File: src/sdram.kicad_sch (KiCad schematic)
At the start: 8 parts, among them U1 ECP5U_12_CABGA256, U10 W9825G6KH-6

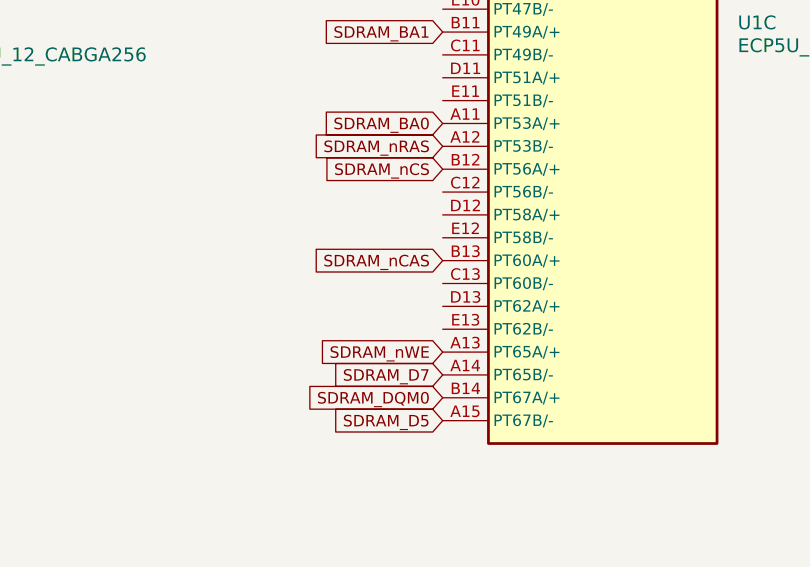
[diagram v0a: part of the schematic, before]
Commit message: Rev 2
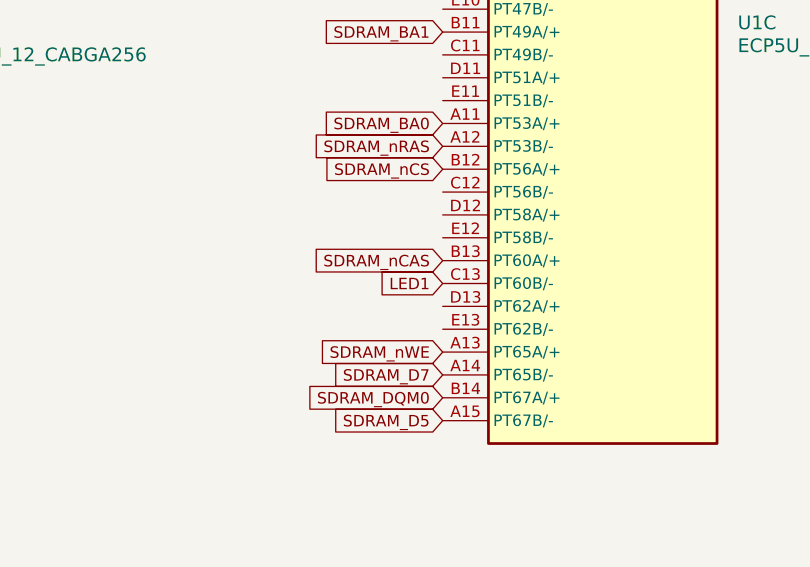
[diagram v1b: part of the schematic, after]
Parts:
- C30, C32: LCSC Part (none) -> C19702
- C31, C33, C34, C35: LCSC Part (none) -> C1525
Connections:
- net LED1: now reaches U1.C13 (PT60B/-)
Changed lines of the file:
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@@
 		)
 	)
+	(global_label "LED1"
+		(shape input)
+		(at 214.63 115.57 180)
+		(effects
+			(font
+				(size 1.27 1.27)
+			)
+			(justify right)
+		)
+		(property "Intersheetrefs" "${INTERSHEET_REFS}"
+			(at 214.63 115.57 0)
+			(effects
+				(font
+					(size 1.27 1.27)
+					(thickness 0.254)
+					(bold yes)
+				)
+				(hide yes)
+			)
+		)
+	)
 	(global_label "SDRAM_A1"
 		(shape input)
@@
 			)
 		)
-		(property "LCSC Part" ""
+		(property "LCSC Part" "C19702"
 			(at 222.25 36.83 0)
 			(effects
@@
 			)
 		)
-		(property "LCSC Part" ""
+		(property "LCSC Part" "C1525"
 			(at 133.35 35.56 0)
 			(effects
@@
 			)
 		)
-		(property "LCSC Part" ""
+		(property "LCSC Part" "C1525"
 			(at 48.26 113.03 0)
 			(effects
@@
 			)
 		)
-		(property "LCSC Part" ""
+		(property "LCSC Part" "C1525"
 			(at 233.68 36.83 0)
 			(effects
@@
 			)
 		)
-		(property "LCSC Part" ""
+		(property "LCSC Part" "C1525"
 			(at 246.38 36.83 0)
 			(effects
@@
 			)
 		)
-		(property "LCSC Part" ""
+		(property "LCSC Part" "C19702"
 			(at 121.92 35.56 0)
 			(effects

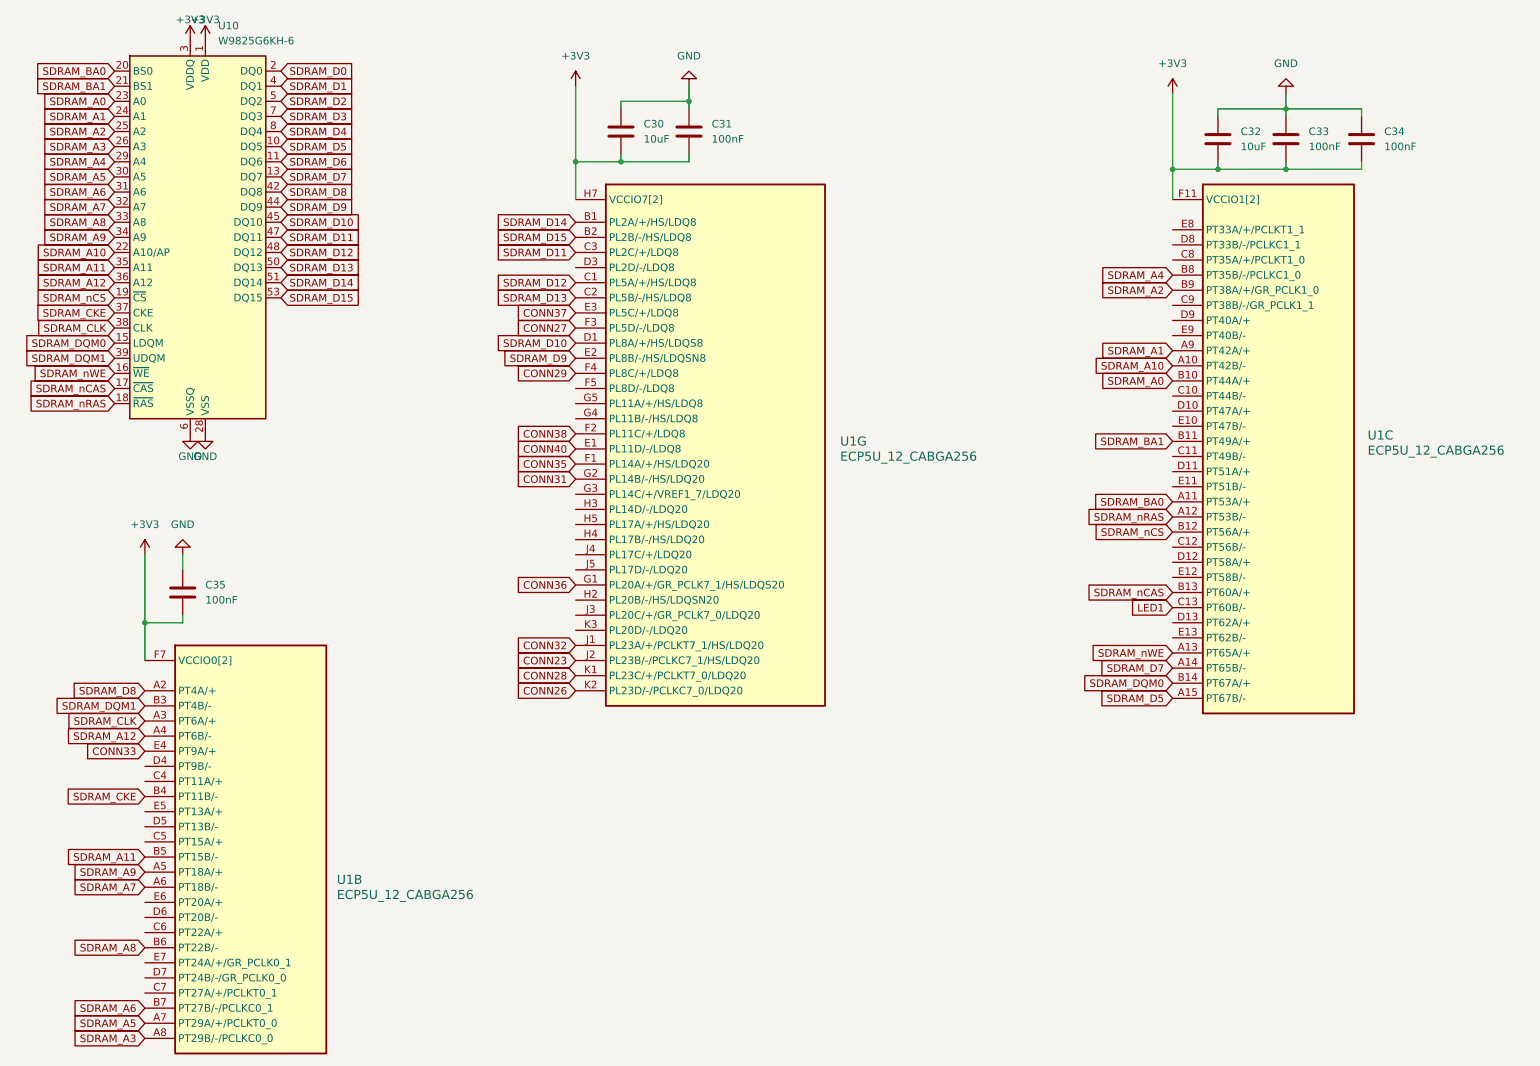
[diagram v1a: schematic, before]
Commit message: Tidy project
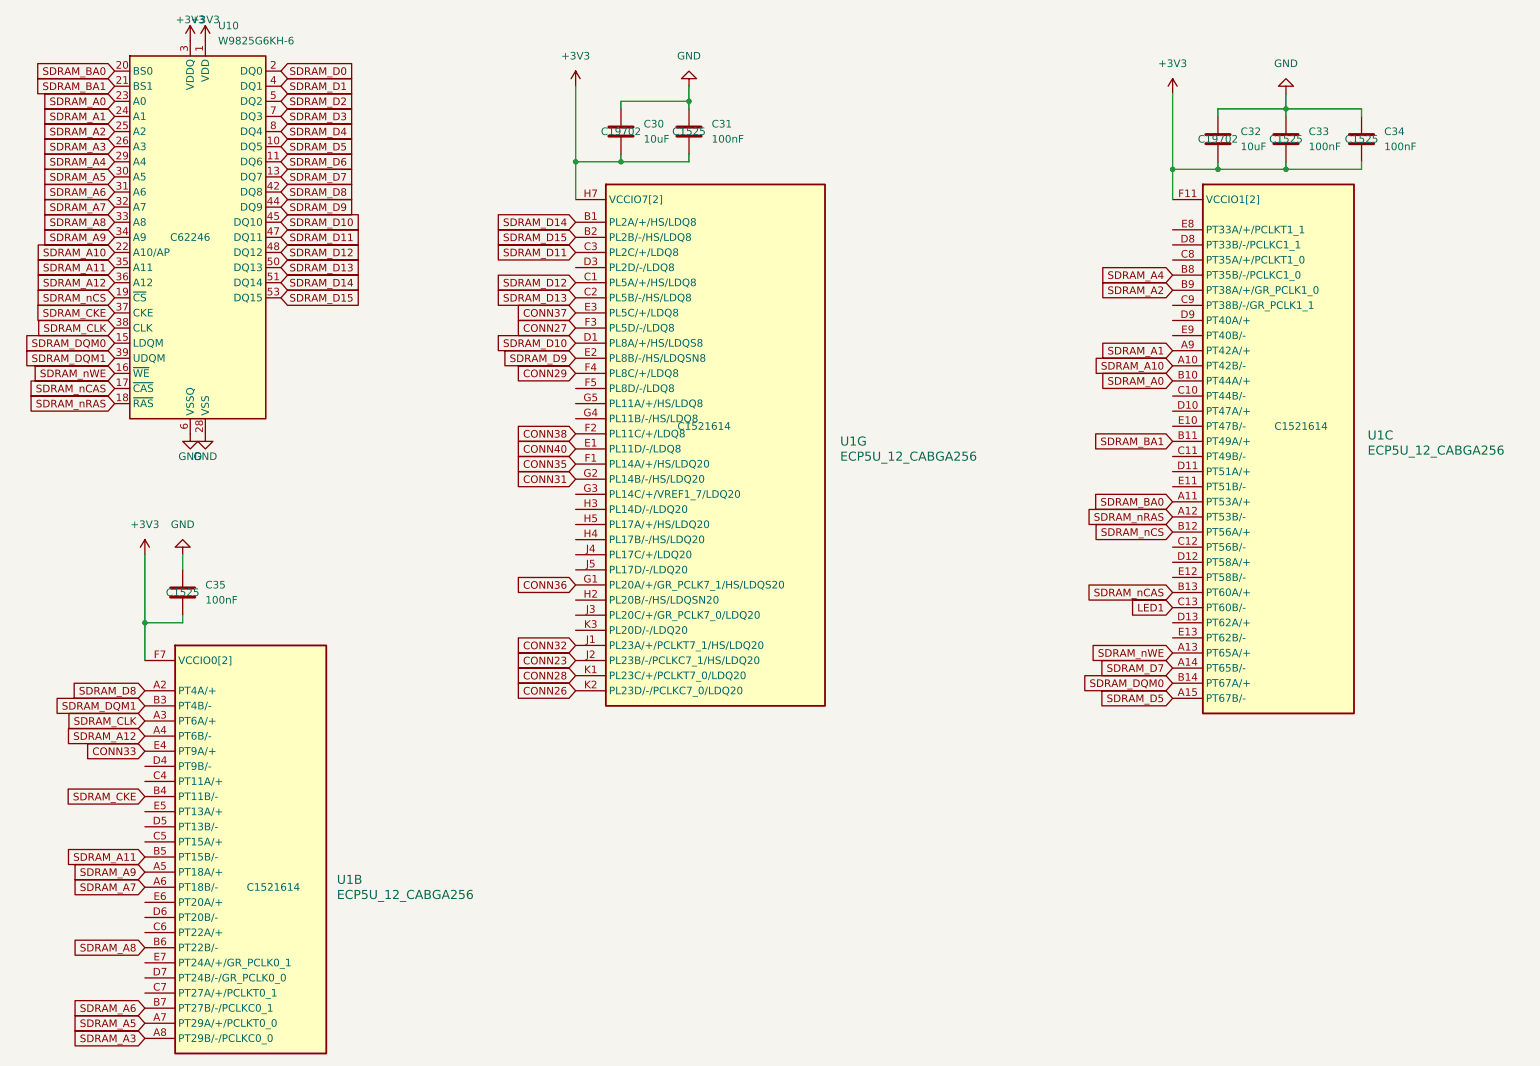
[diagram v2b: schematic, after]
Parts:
- C30, C32: JLCPCB Part # (none) -> C19702; LCSC Part C19702 -> (none)
- C31, C33, C34, C35: JLCPCB Part # (none) -> C1525; LCSC Part C1525 -> (none)
- U1: JLCPCB Part # (none) -> C1521614; LCSC Part C1521614 -> (none)
- U10: JLCPCB Part # (none) -> C62246; LCSC Part C62246 -> (none)
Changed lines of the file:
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@@
 			)
 		)
-		(property "LCSC Part" "C19702"
+		(property "JLCPCB Part #" "C19702"
 			(at 222.25 36.83 0)
 			(effects
@@
 					(size 1.27 1.27)
 				)
-				(hide yes)
 			)
 		)
@@
 			)
 		)
-		(property "LCSC Part" " C1521614"
+		(property "JLCPCB Part #" " C1521614"
 			(at 236.22 85.09 0)
 			(effects
@@
 					(size 1.27 1.27)
 				)
-				(hide yes)
 			)
 		)
@@
 			)
 		)
-		(property "LCSC Part" " C1521614"
+		(property "JLCPCB Part #" " C1521614"
 			(at 63.5 162.56 0)
 			(effects
@@
 					(size 1.27 1.27)
 				)
-				(hide yes)
 			)
 		)
@@
 			)
 		)
-		(property "LCSC Part" " C62246"
+		(property "JLCPCB Part #" " C62246"
 			(at 49.53 53.34 0)
 			(effects
@@
 					(size 1.27 1.27)
 				)
-				(hide yes)
 			)
 		)
@@
 			)
 		)
-		(property "LCSC Part" "C1525"
+		(property "JLCPCB Part #" "C1525"
 			(at 133.35 35.56 0)
 			(effects
@@
 					(size 1.27 1.27)
 				)
-				(hide yes)
 			)
 		)
@@
 			)
 		)
-		(property "LCSC Part" "C1525"
+		(property "JLCPCB Part #" "C1525"
 			(at 48.26 113.03 0)
 			(effects
@@
 					(size 1.27 1.27)
 				)
-				(hide yes)
 			)
 		)
@@
 			)
 		)
-		(property "LCSC Part" "C1525"
+		(property "JLCPCB Part #" "C1525"
 			(at 233.68 36.83 0)
 			(effects
@@
 					(size 1.27 1.27)
 				)
-				(hide yes)
 			)
 		)
@@
 			)
 		)
-		(property "LCSC Part" " C1521614"
+		(property "JLCPCB Part #" " C1521614"
 			(at 135.89 85.09 0)
 			(effects
@@
 					(size 1.27 1.27)
 				)
-				(hide yes)
 			)
 		)
@@
 			)
 		)
-		(property "LCSC Part" "C1525"
+		(property "JLCPCB Part #" "C1525"
 			(at 246.38 36.83 0)
 			(effects
@@
 					(size 1.27 1.27)
 				)
-				(hide yes)
 			)
 		)
@@
 			)
 		)
-		(property "LCSC Part" "C19702"
+		(property "JLCPCB Part #" "C19702"
 			(at 121.92 35.56 0)
 			(effects
@@
 					(size 1.27 1.27)
 				)
-				(hide yes)
-			)
-		)
+			)
+		)
